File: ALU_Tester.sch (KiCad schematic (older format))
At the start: 15 parts, among them J1 Conn_02x18_Odd_Even, J2 Conn_01x02, SW1 SW_SPST, U1 74LS181, U2 74LS181

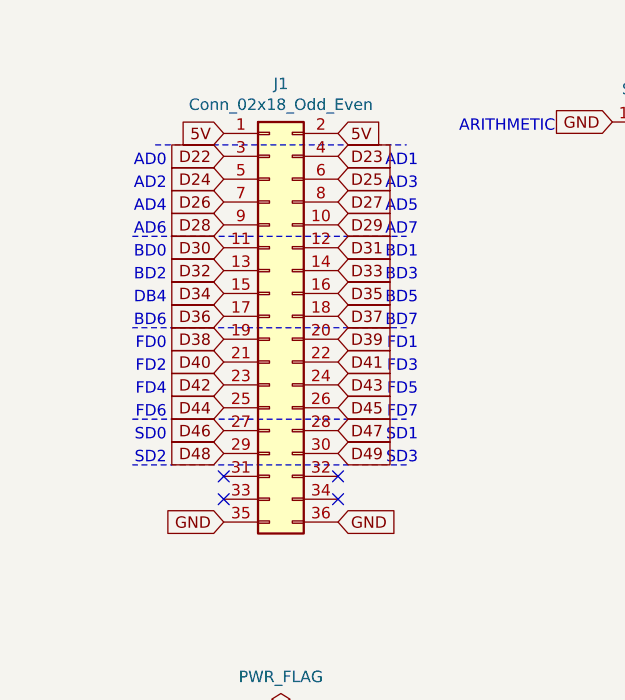
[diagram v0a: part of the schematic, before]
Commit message: Daily Update
Added code to project.
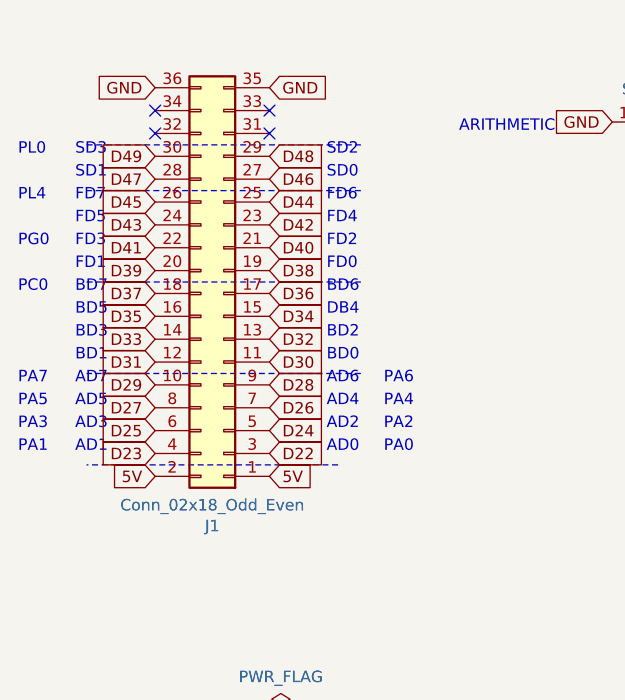
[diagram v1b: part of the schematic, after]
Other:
- note added: "PA0"
- note added: "PA1"
- note added: "PA2"
- note added: "PA3"
- note added: "PA4"
- note added: "PA5"
- note added: "PA6"
- note added: "PA7"
- note added: "PC0"
- note added: "PG0"
- note added: "PL0"
- note added: "PL4"
- moved on the sheet: J1
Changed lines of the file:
@@
 L Connector_Generic:Conn_02x18_Odd_Even J1
 U 1 1 5E9A59D8
-P 2200 3850
-F 0 "J1" H 2250 4867 50  0000 C CNN
-F 1 "Conn_02x18_Odd_Even" H 2250 4776 50  0000 C CNN
-F 2 "Connector_PinHeader_2.54mm:PinHeader_2x18_P2.54mm_Vertical" H 2200 3850 50  0001 C CNN
-F 3 "~" H 2200 3850 50  0001 C CNN
-	1    2200 3850
-	1    0    0    -1
-$EndComp
-Text GLabel 2000 3050 0    50   Input ~ 0
-5V
-Text GLabel 2500 3050 2    50   Input ~ 0
-5V
-Text GLabel 2000 4750 0    50   Input ~ 0
+P 2000 3750
+F 0 "J1" H 2050 4767 50  0000 C CNN
+F 1 "Conn_02x18_Odd_Even" H 2050 4676 50  0000 C CNN
+F 2 "Connector_PinHeader_2.54mm:PinHeader_2x18_P2.54mm_Vertical" H 2000 3750 50  0001 C CNN
+F 3 "~" H 2000 3750 50  0001 C CNN
+	1    2000 3750
+	-1   0    0    1
+$EndComp
+Text GLabel 2200 4550 2    50   Input ~ 0
+5V
+Text GLabel 1700 4550 0    50   Input ~ 0
+5V
+Text GLabel 2200 2850 2    50   Input ~ 0
 GND
-Text GLabel 2500 4750 2    50   Input ~ 0
+Text GLabel 1700 2850 0    50   Input ~ 0
 GND
-Text GLabel 2000 3150 0    50   Input ~ 0
+Text GLabel 2200 4450 2    50   Input ~ 0
 D22
-Text GLabel 2000 3250 0    50   Input ~ 0
+Text GLabel 2200 4350 2    50   Input ~ 0
 D24
-Text GLabel 2000 3350 0    50   Input ~ 0
+Text GLabel 2200 4250 2    50   Input ~ 0
 D26
-Text GLabel 2000 3450 0    50   Input ~ 0
+Text GLabel 2200 4150 2    50   Input ~ 0
 D28
-Text GLabel 2000 3550 0    50   Input ~ 0
+Text GLabel 2200 4050 2    50   Input ~ 0
 D30
-Text GLabel 2000 3650 0    50   Input ~ 0
+Text GLabel 2200 3950 2    50   Input ~ 0
 D32
-Text GLabel 2000 3750 0    50   Input ~ 0
+Text GLabel 2200 3850 2    50   Input ~ 0
 D34
-Text GLabel 2000 3850 0    50   Input ~ 0
+Text GLabel 2200 3750 2    50   Input ~ 0
 D36
-Text GLabel 2000 3950 0    50   Input ~ 0
+Text GLabel 2200 3650 2    50   Input ~ 0
 D38
-Text GLabel 2000 4050 0    50   Input ~ 0
+Text GLabel 2200 3550 2    50   Input ~ 0
 D40
-Text GLabel 2000 4150 0    50   Input ~ 0
+Text GLabel 2200 3450 2    50   Input ~ 0
 D42
-Text GLabel 2000 4250 0    50   Input ~ 0
+Text GLabel 2200 3350 2    50   Input ~ 0
 D44
-Text GLabel 2000 4350 0    50   Input ~ 0
+Text GLabel 2200 3250 2    50   Input ~ 0
 D46
-Text GLabel 2000 4450 0    50   Input ~ 0
+Text GLabel 2200 3150 2    50   Input ~ 0
 D48
-Text GLabel 2500 3150 2    50   Input ~ 0
+Text GLabel 1700 4450 0    50   Input ~ 0
 D23
-Text GLabel 2500 3250 2    50   Input ~ 0
+Text GLabel 1700 4350 0    50   Input ~ 0
 D25
-Text GLabel 2500 3350 2    50   Input ~ 0
+Text GLabel 1700 4250 0    50   Input ~ 0
 D27
-Text GLabel 2500 3450 2    50   Input ~ 0
+Text GLabel 1700 4150 0    50   Input ~ 0
 D29
-Text GLabel 2500 3550 2    50   Input ~ 0
+Text GLabel 1700 4050 0    50   Input ~ 0
 D31
-Text GLabel 2500 3650 2    50   Input ~ 0
+Text GLabel 1700 3950 0    50   Input ~ 0
 D33
-Text GLabel 2500 3750 2    50   Input ~ 0
+Text GLabel 1700 3850 0    50   Input ~ 0
 D35
-Text GLabel 2500 3850 2    50   Input ~ 0
+Text GLabel 1700 3750 0    50   Input ~ 0
 D37
-Text GLabel 2500 3950 2    50   Input ~ 0
+Text GLabel 1700 3650 0    50   Input ~ 0
 D39
-Text GLabel 2500 4050 2    50   Input ~ 0
+Text GLabel 1700 3550 0    50   Input ~ 0
 D41
-Text GLabel 2500 4150 2    50   Input ~ 0
+Text GLabel 1700 3450 0    50   Input ~ 0
 D43
-Text GLabel 2500 4250 2    50   Input ~ 0
+Text GLabel 1700 3350 0    50   Input ~ 0
 D45
-Text GLabel 2500 4350 2    50   Input ~ 0
+Text GLabel 1700 3250 0    50   Input ~ 0
 D47
-Text GLabel 2500 4450 2    50   Input ~ 0
+Text GLabel 1700 3150 0    50   Input ~ 0
 D49
 $Comp
@@
 	4250 2600 4450 2600
 Wire Notes Line
-	1700 3100 2800 3100
+	2500 4500 1400 4500
 Wire Notes Line
-	1600 3500 2800 3500
+	2600 4100 1400 4100
 Wire Notes Line
-	2800 3900 1600 3900
+	1400 3700 2600 3700
 Wire Notes Line
-	1600 4300 2800 4300
+	2600 3300 1400 3300
 Wire Notes Line
-	2800 4500 1600 4500
-Text Notes 1750 3200 2    50   ~ 0
+	1400 3100 2600 3100
+Text Notes 2450 4450 0    50   ~ 0
 AD0
-Text Notes 1750 3600 2    50   ~ 0
+Text Notes 2450 4050 0    50   ~ 0
 BD0
-Text Notes 1750 4000 2    50   ~ 0
+Text Notes 2450 3650 0    50   ~ 0
 FD0
-Text Notes 1750 4400 2    50   ~ 0
+Text Notes 2450 3250 0    50   ~ 0
 SD0
-Text Notes 1750 3300 2    50   ~ 0
+Text Notes 2450 4350 0    50   ~ 0
 AD2
-Text Notes 1750 3400 2    50   ~ 0
+Text Notes 2450 4250 0    50   ~ 0
 AD4
-Text Notes 1750 3500 2    50   ~ 0
+Text Notes 2450 4150 0    50   ~ 0
 AD6
-Text Notes 1750 3700 2    50   ~ 0
+Text Notes 2450 3950 0    50   ~ 0
 BD2
-Text Notes 1750 3800 2    50   ~ 0
+Text Notes 2450 3850 0    50   ~ 0
 DB4
-Text Notes 1750 3900 2    50   ~ 0
+Text Notes 2450 3750 0    50   ~ 0
 BD6
-Text Notes 1750 4100 2    50   ~ 0
+Text Notes 2450 3550 0    50   ~ 0
 FD2
-Text Notes 1750 4200 2    50   ~ 0
+Text Notes 2450 3450 0    50   ~ 0
 FD4
-Text Notes 1750 4300 2    50   ~ 0
+Text Notes 2450 3350 0    50   ~ 0
 FD6
-Text Notes 2850 3200 2    50   ~ 0
+Text Notes 1350 4450 0    50   ~ 0
 AD1
-Text Notes 2850 3300 2    50   ~ 0
+Text Notes 1350 4350 0    50   ~ 0
 AD3
-Text Notes 2850 3400 2    50   ~ 0
+Text Notes 1350 4250 0    50   ~ 0
 AD5
-Text Notes 2850 3500 2    50   ~ 0
+Text Notes 1350 4150 0    50   ~ 0
 AD7
-Text Notes 2850 3600 2    50   ~ 0
+Text Notes 1350 4050 0    50   ~ 0
 BD1
-Text Notes 2850 3700 2    50   ~ 0
+Text Notes 1350 3950 0    50   ~ 0
 BD3
-Text Notes 2850 3800 2    50   ~ 0
+Text Notes 1350 3850 0    50   ~ 0
 BD5
-Text Notes 2850 3900 2    50   ~ 0
+Text Notes 1350 3750 0    50   ~ 0
 BD7
-Text Notes 2850 4000 2    50   ~ 0
+Text Notes 1350 3650 0    50   ~ 0
 FD1
-Text Notes 2850 4100 2    50   ~ 0
+Text Notes 1350 3550 0    50   ~ 0
 FD3
-Text Notes 2850 4200 2    50   ~ 0
+Text Notes 1350 3450 0    50   ~ 0
 FD5
-Text Notes 2850 4300 2    50   ~ 0
+Text Notes 1350 3350 0    50   ~ 0
 FD7
-Text Notes 1750 4500 2    50   ~ 0
+Text Notes 2450 3150 0    50   ~ 0
 SD2
-Text Notes 2850 4500 2    50   ~ 0
+Text Notes 1350 3150 0    50   ~ 0
 SD3
-Text Notes 2850 4400 2    50   ~ 0
+Text Notes 1350 3250 0    50   ~ 0
 SD1
-NoConn ~ 2000 4550
-NoConn ~ 2000 4650
-NoConn ~ 2500 4650
-NoConn ~ 2500 4550
+NoConn ~ 2200 3050
+NoConn ~ 2200 2950
+NoConn ~ 1700 2950
+NoConn ~ 1700 3050
 NoConn ~ 6950 4450
 NoConn ~ 6950 4350
@@
 Wire Wire Line
 	4350 7100 4150 7100
+Text Notes 1100 4450 0    50   ~ 0
+PA1
+Text Notes 2700 4450 0    50   ~ 0
+PA0
+Text Notes 1100 4350 0    50   ~ 0
+PA3
+Text Notes 1100 4250 0    50   ~ 0
+PA5
+Text Notes 1100 4150 0    50   ~ 0
+PA7
+Text Notes 2700 4350 0    50   ~ 0
+PA2
+Text Notes 2700 4250 0    50   ~ 0
+PA4
+Text Notes 2700 4150 0    50   ~ 0
+PA6
+Text Notes 1100 3750 0    50   ~ 0
+PC0
+Text Notes 1100 3550 0    50   ~ 0
+PG0
+Text Notes 1100 3350 0    50   ~ 0
+PL4
+Text Notes 1100 3150 0    50   ~ 0
+PL0
 $EndSCHEMATC
